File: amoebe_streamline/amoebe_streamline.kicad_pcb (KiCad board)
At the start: 2 copper layers, 19.1 x 19 mm, 11 parts, among them J1 Conn_01x02_Pin, J2 Conn_01x02_Pin, J3 Conn_01x02_Pin, J4 Conn_01x02_Pin, J5 Conn_01x02_Pin, J6 Conn_01x02_Pin

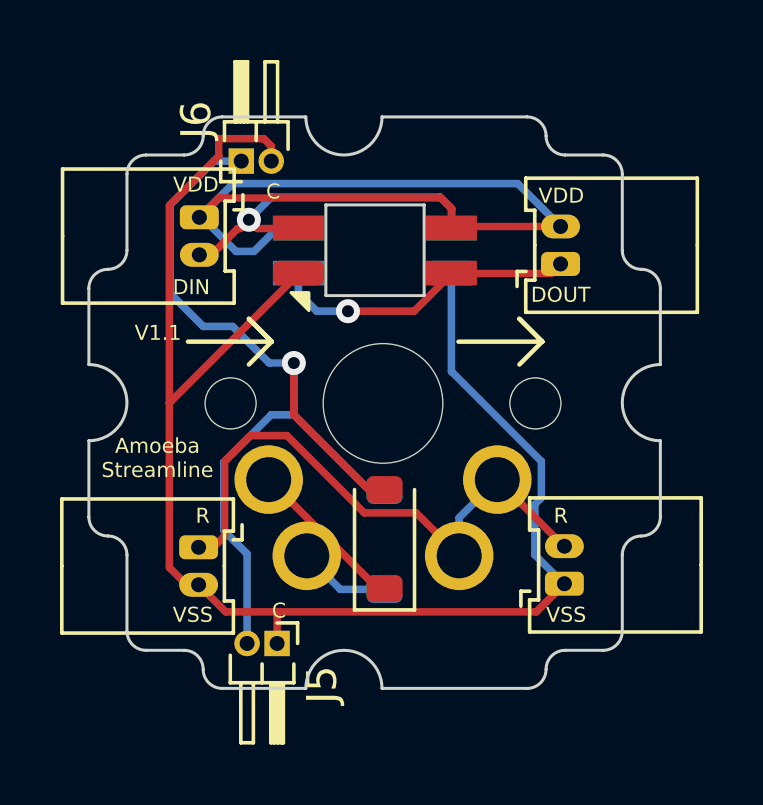
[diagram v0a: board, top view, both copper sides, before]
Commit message: updated pcb design
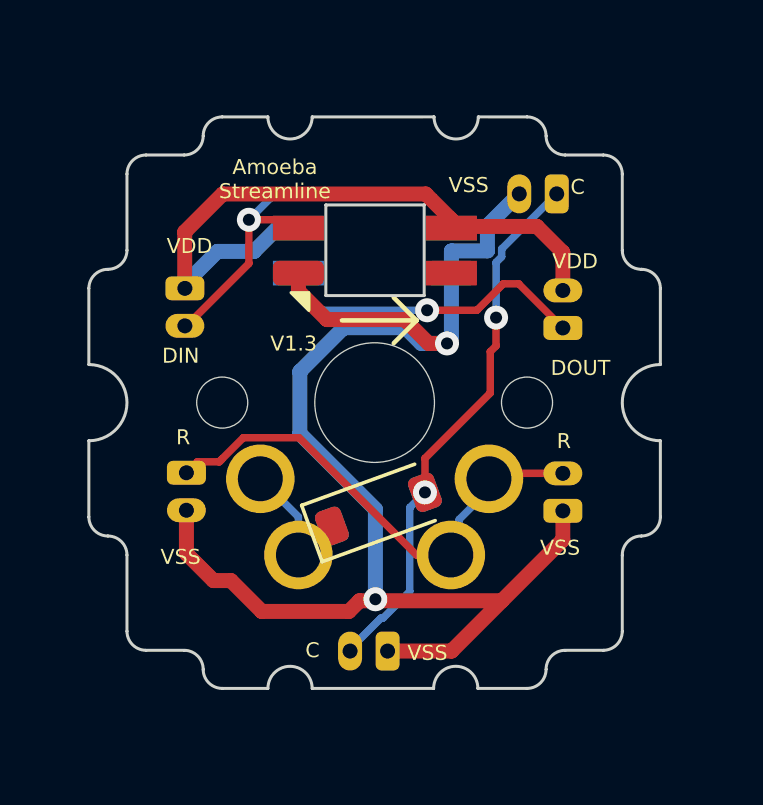
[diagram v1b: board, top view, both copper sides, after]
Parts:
- J1, J2, J3, J4: footprint Connector_Molex:Molex_PicoBlade_53048-0210_1x02_P1.25mm_Horizontal -> Connector_Molex:Molex_PicoBlade_53047-0210_1x02_P1.25mm_Vertical
- J5, J6: footprint Connector_PinHeader_1.00mm:PinHeader_1x02_P1.00mm_Horizontal -> Connector_Molex:Molex_PicoBlade_53047-0210_1x02_P1.25mm_Vertical
- moved J6 10.6 mm to (148.9, 93.4), turned to 180 degrees
- moved J5 3.69 mm to (143.3, 108.6), turned to 180 degrees
- moved J4 2.52 mm to (136.6, 102.7)
- moved J2 2.43 mm to (149.1, 103.9)
- moved J1 2.42 mm to (136.6, 96.5)
- moved J3 2.13 mm to (149.1, 97.8)
- moved D1 1.04 mm to (143.0, 103.9), turned to 20 degrees
- moved D1 1.01 mm to (143.0, 103.9), turned to 20 degrees
- moved S1 0.28 mm to (142.9, 100.3)
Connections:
- S1 pad : (no net) -> Net-(D1-A)
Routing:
- net /C: track 31.4 -> 18.1 mm, vias 1 -> 2
- net /VDD: track 30.4 -> 21.6 mm
- net Net-(D1-A): track 8.42 -> 3.07 mm
- net /R: track 19.6 -> 16.6 mm
- net /VSS: track 50.9 -> 48.7 mm, vias 0 -> 2
- net /DIN: track 11.8 -> 13.9 mm
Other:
- board size 19.1 x 19 mm -> 19.1 x 19.1 mm
- board text added: "V1.3"
- board text removed: "V1.1"
